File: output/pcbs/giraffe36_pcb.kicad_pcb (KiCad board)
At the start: 2 copper layers, 127.5 x 120.6 mm, 20 parts

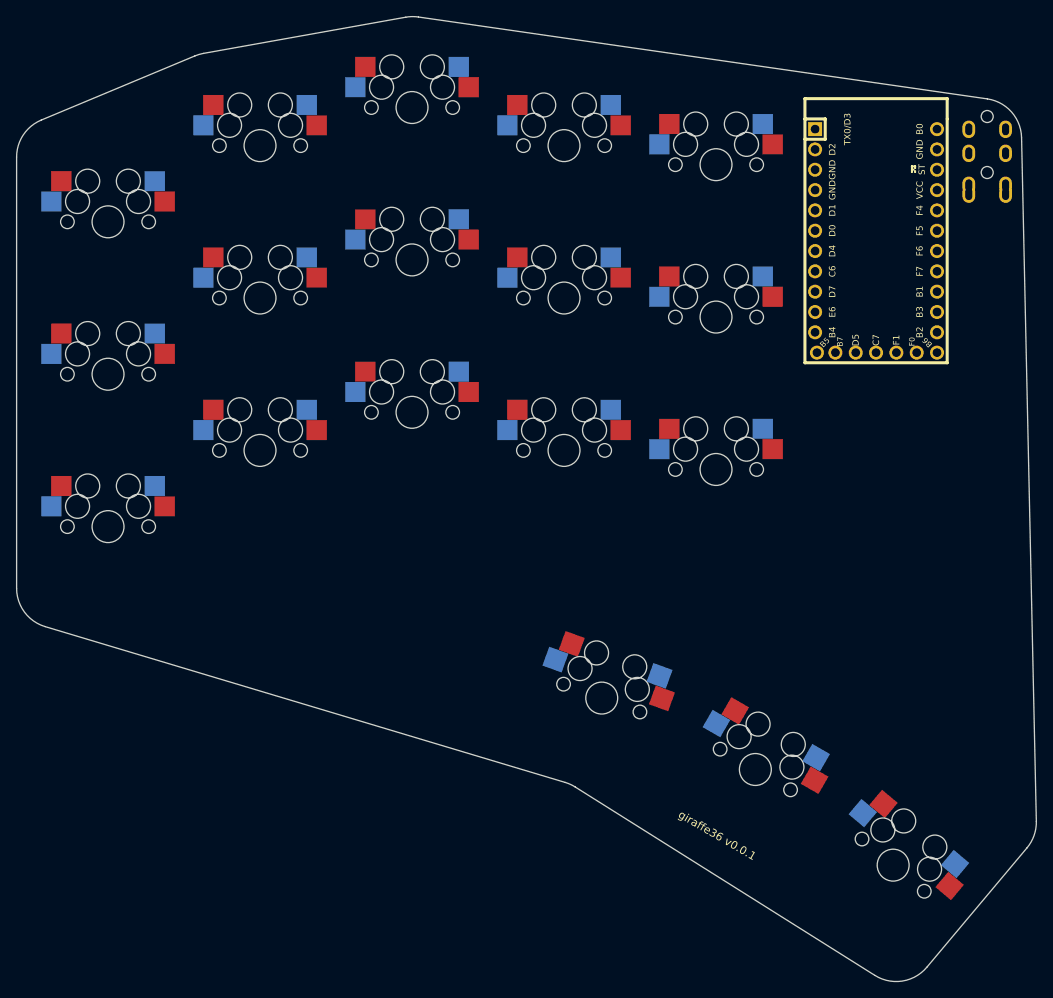
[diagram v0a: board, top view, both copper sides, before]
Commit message: tweak outlines and routing
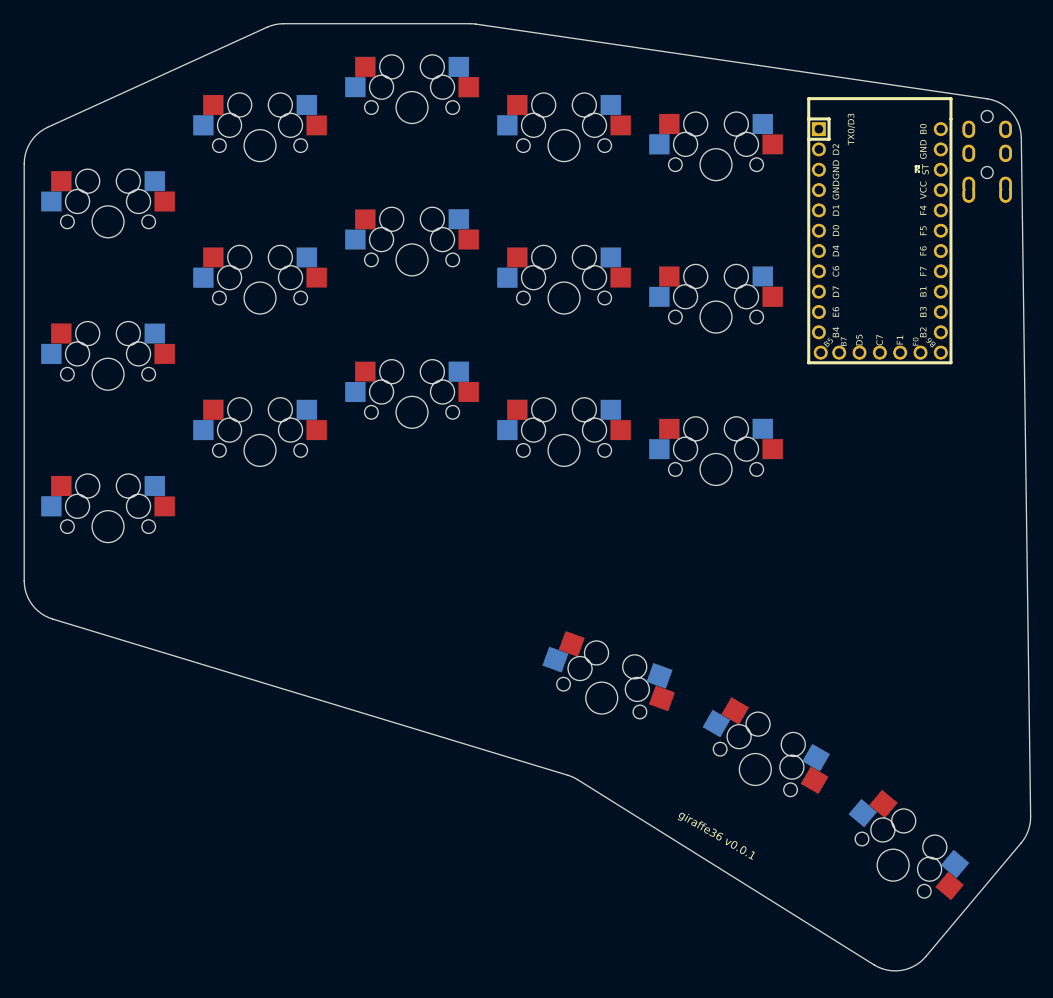
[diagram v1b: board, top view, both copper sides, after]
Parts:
- moved ? 0.48 mm to (248.9, 116.7)
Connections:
- ? pad 10: matrix_middle_home -> matrix_inner_home
- ? pad 8: matrix_index_home -> matrix_middle_home
- ? pad 9: matrix_inner_home -> matrix_index_home
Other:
- board size 127.5 x 120.6 mm -> 125.8 x 118.4 mm
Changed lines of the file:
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@@
         )
     (module "Elite-C" (layer "F.Cu")
-      (at 248.4025 116.68125 270)
+      (at 248.87875 116.68125 270)
       (attr through_hole)
       (fp_text value "Elite-C" (at 0 0) (layer "F.SilkS") hide
@@
       (pad "6" thru_hole circle (at -1.27 7.62) (size 1.7526 1.7526) (drill 1.0922) (layers *.Cu *.SilkS *.Mask) (net 7 "matrix_ring_top"))
       (pad "7" thru_hole circle (at 1.27 7.62) (size 1.7526 1.7526) (drill 1.0922) (layers *.Cu *.SilkS *.Mask) (net 4 "matrix_pinky_top"))
-      (pad "8" thru_hole circle (at 3.81 7.62) (size 1.7526 1.7526) (drill 1.0922) (layers *.Cu *.SilkS *.Mask) (net 12 "matrix_index_home"))
-      (pad "9" thru_hole circle (at 6.35 7.62) (size 1.7526 1.7526) (drill 1.0922) (layers *.Cu *.SilkS *.Mask) (net 15 "matrix_inner_home"))
-      (pad "10" thru_hole circle (at 8.89 7.62) (size 1.7526 1.7526) (drill 1.0922) (layers *.Cu *.SilkS *.Mask) (net 9 "matrix_middle_home"))
+      (pad "8" thru_hole circle (at 3.81 7.62) (size 1.7526 1.7526) (drill 1.0922) (layers *.Cu *.SilkS *.Mask) (net 9 "matrix_middle_home"))
+      (pad "9" thru_hole circle (at 6.35 7.62) (size 1.7526 1.7526) (drill 1.0922) (layers *.Cu *.SilkS *.Mask) (net 12 "matrix_index_home"))
+      (pad "10" thru_hole circle (at 8.89 7.62) (size 1.7526 1.7526) (drill 1.0922) (layers *.Cu *.SilkS *.Mask) (net 15 "matrix_inner_home"))
       (pad "11" thru_hole circle (at 11.43 7.62) (size 1.7526 1.7526) (drill 1.0922) (layers *.Cu *.SilkS *.Mask) (net 6 "matrix_ring_home"))
       (pad "12" thru_hole circle (at 13.97 7.3914) (size 1.7526 1.7526) (drill 1.0922) (layers *.Cu *.SilkS *.Mask) (net 3 "matrix_pinky_home"))
@@
                 (effects (font (size 1 1) (thickness 0.15)) )
             )
-            (gr_line (start 268.43787433146827 189.2364429923946) (end 266.5915397481229 103.7734355283701) (angle 90) (layer Edge.Cuts) (width 0.15))
-(gr_line (start 262.3050591786624 98.93243484859755) (end 191.1986430372401 88.69745579722957) (angle 90) (layer Edge.Cuts) (width 0.15))
-(gr_line (start 189.6057370284023 88.72459907596672) (end 164.31994965775277 93.24839931461129) (angle 90) (layer Edge.Cuts) (width 0.15))
-(gr_line (start 163.2738356048592 93.55636413256097) (end 144.04333296444227 101.58663759376094) (angle 90) (layer Edge.Cuts) (width 0.15))
-(gr_line (start 140.97 106.20052467891279) (end 140.97 160.10840398922608) (angle 90) (layer Edge.Cuts) (width 0.15))
-(gr_line (start 144.5350394450162 164.8980686727532) (end 209.55217616364516 184.37689015349645) (angle 90) (layer Edge.Cuts) (width 0.15))
-(gr_line (start 210.77856208033032 184.93367938208416) (end 248.2577161049487 208.4980418824439) (angle 90) (layer Edge.Cuts) (width 0.15))
-(gr_line (start 254.74928474322292 207.4791045673029) (end 267.2692629024389 192.55837563426132) (angle 90) (layer Edge.Cuts) (width 0.15))
-(gr_arc (start 261.5927061524883 103.88143003043842) (end 266.5915397524883 103.77343553043842) (angle -80.57154310169524) (layer Edge.Cuts) (width 0.15))
-(gr_arc (start 190.48629001106642 93.64645097906825) (end 191.19864301106642 88.69745577906825) (angle -18.334129319859528) (layer Edge.Cuts) (width 0.15))
-(gr_arc (start 165.20050264041691 98.1702512177128) (end 164.31994964041692 93.2483993177128) (angle -12.521145693837937) (layer Edge.Cuts) (width 0.15))
-(gr_arc (start 145.97 106.20052467891279) (end 144.043333 101.58663757891279) (angle -67.3355598115637) (layer Edge.Cuts) (width 0.15))
-(gr_arc (start 145.97 160.10840398922608) (end 140.97 160.10840398922608) (angle -73.32203635384576) (layer Edge.Cuts) (width 0.15))
-(gr_arc (start 208.11721560866138 189.1665548370236) (end 210.7785621086614 184.9336793370236) (angle -15.480947111767009) (layer Edge.Cuts) (width 0.15))
-(gr_arc (start 250.91906257661768 204.26516642750448) (end 248.25771607661767 208.4980419275045) (angle -82.1589095950444) (layer Edge.Cuts) (width 0.15))
-(gr_arc (start 263.4390407358337 189.34443749446302) (end 267.2692629358337 192.55837559446303) (angle -41.23762323591903) (layer Edge.Cuts) (width 0.15))
+            (gr_line (start 267.7233337781094 188.64636047823296) (end 266.5585210459172 103.79904152942254) (angle 90) (layer Edge.Cuts) (width 0.15))
+(gr_line (start 262.28155811664254 98.92016220960969) (end 198.37937702494528 89.58748568152359) (angle 90) (layer Edge.Cuts) (width 0.15))
+(gr_line (start 197.6568110514561 89.53500000000003) (end 174.34119148542428 89.53500000000003) (angle 90) (layer Edge.Cuts) (width 0.15))
+(gr_line (start 172.26670854038835 89.98565712053627) (end 144.84801705496412 102.48847542734222) (angle 90) (layer Edge.Cuts) (width 0.15))
+(gr_line (start 141.9225 107.037818306806) (end 141.9225 159.16861772182457) (angle 90) (layer Edge.Cuts) (width 0.15))
+(gr_line (start 145.47185401934755 163.95355515800708) (end 209.89369569872298 183.48427952349323) (angle 90) (layer Edge.Cuts) (width 0.15))
+(gr_line (start 211.09200633600454 184.02857677087837) (end 248.14444404538048 207.17373776925433) (angle 90) (layer Edge.Cuts) (width 0.15))
+(gr_line (start 254.62362278067937 206.14703567893775) (end 266.5540269927103 191.92893357538117) (angle 90) (layer Edge.Cuts) (width 0.15))
+(gr_arc (start 261.5589921431532 103.86767652808703) (end 266.5585210431532 103.79904152808703) (angle -80.90438567212655) (layer Edge.Cuts) (width 0.15))
+(gr_arc (start 197.6568110514561 94.53500000000003) (end 198.3793770514561 89.58748560000002) (angle -8.309090475830658) (layer Edge.Cuts) (width 0.15))
+(gr_arc (start 174.34119148542428 94.53500000000003) (end 174.34119148542428 89.53500000000003) (angle -24.5128043054565) (layer Edge.Cuts) (width 0.15))
+(gr_arc (start 146.9225 107.037818306806) (end 144.84801710000002 102.488475406806) (angle -65.48719569454393) (layer Edge.Cuts) (width 0.15))
+(gr_arc (start 146.9225 159.16861772182457) (end 141.9225 159.16861772182457) (angle -73.1343090469096) (layer Edge.Cuts) (width 0.15))
+(gr_arc (start 208.4430497180705 188.2692169596757) (end 211.0920063180705 184.0285767596757) (angle -15.125665267156585) (layer Edge.Cuts) (width 0.15))
+(gr_arc (start 250.7934006633145 202.933097580457) (end 248.1444440633145 207.173737780457) (angle -81.99135505737092) (layer Edge.Cuts) (width 0.15))
+(gr_arc (start 262.7238048753455 188.7149954769004) (end 266.55402707534546 191.92893357690042) (angle -40.786525014952915) (layer Edge.Cuts) (width 0.15))
 )
